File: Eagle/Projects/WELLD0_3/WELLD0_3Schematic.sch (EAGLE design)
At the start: 9 parts

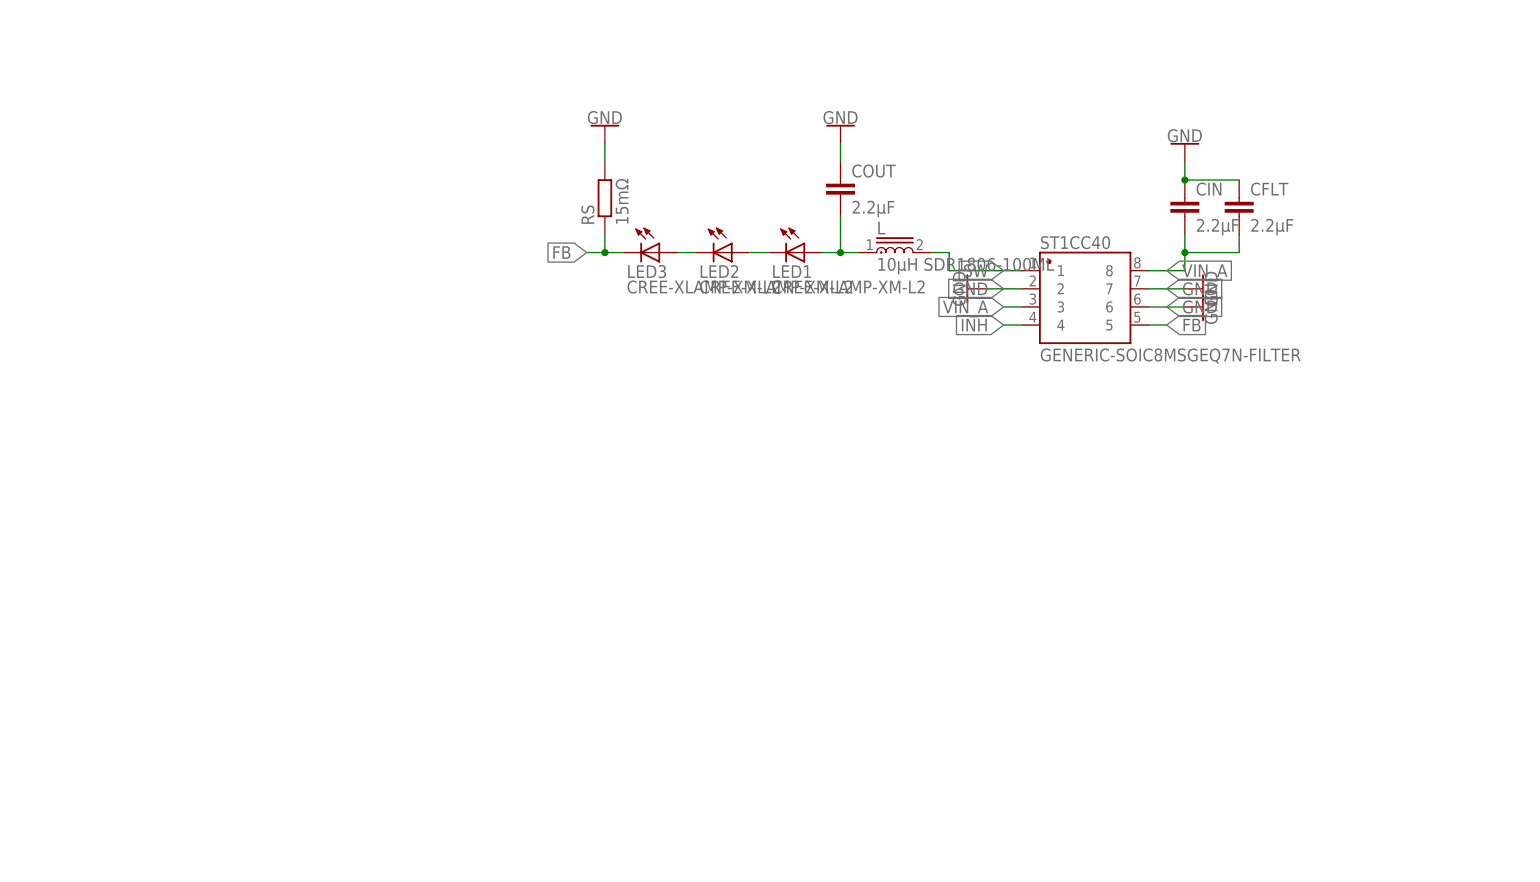
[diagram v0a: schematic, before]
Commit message: Work from 16/10-18
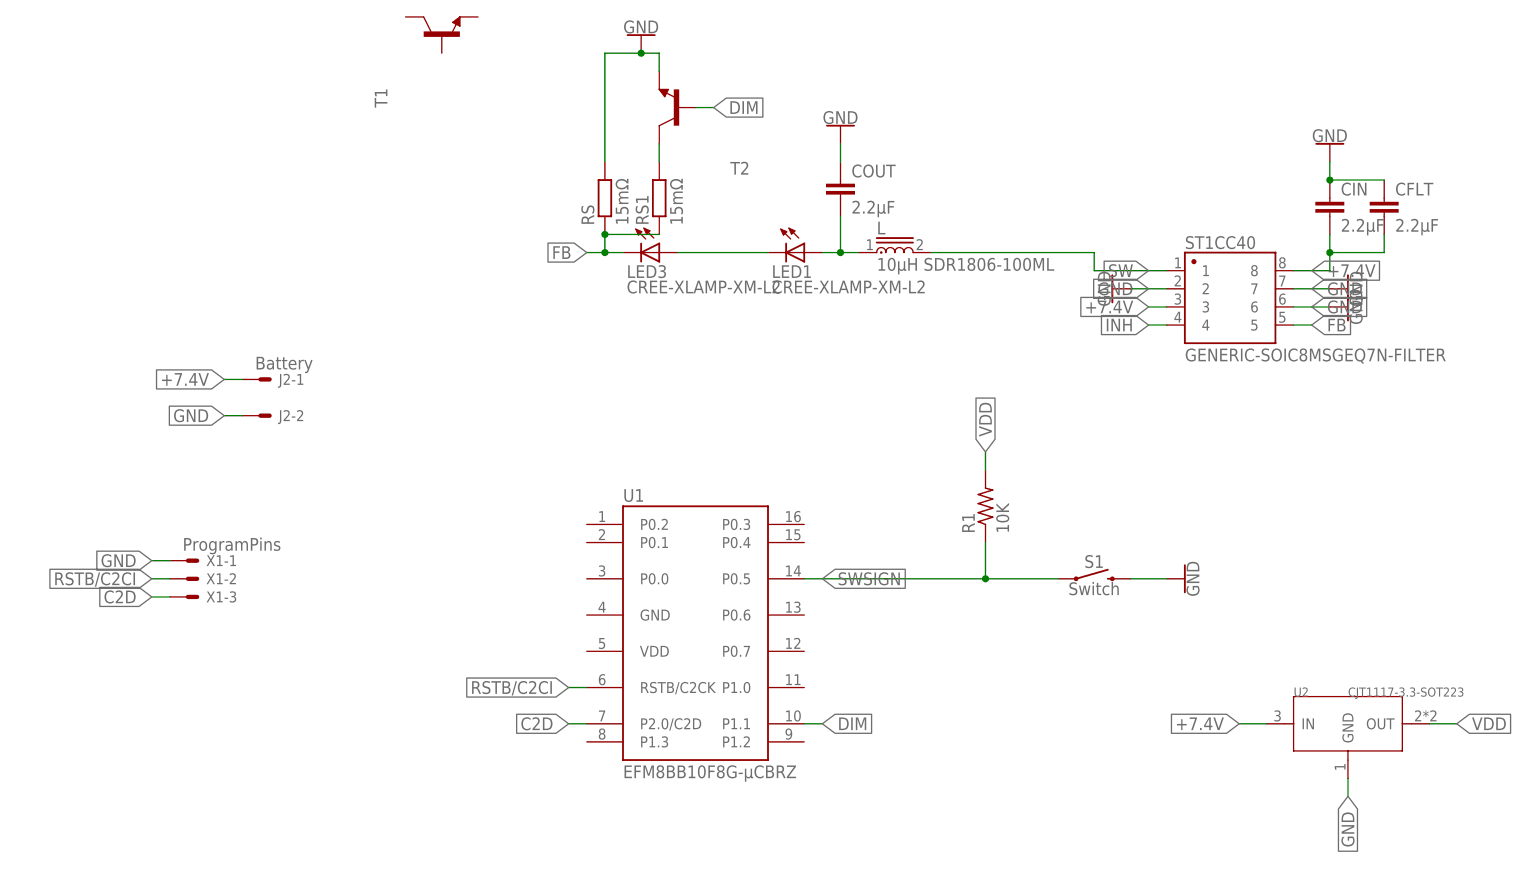
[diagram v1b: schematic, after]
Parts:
- removed LED2: CREE-XLAMP-XM-L2, led:CREE-XLAMP-XM-L
- added J2: Battery, con-molex:22-27-2021-02
- added R1: 10K, audio amplifier example:R-US_R0603
- added RS1: 15mΩ, rcl:R-EU_M1206
- added S1: Switch, SparkFun-Switches:MOMENTARY-SWITCH-SPST-SMD-6.2MM-TALL
- added T1, T2: (no value), DC_LOAD_AU:-NPN-SOT23-BEC
- added U1: EFM8BB10F8G-µCBRZ, adg451_adg452_adg453:EFM8BB10F8G-µCBRZ
- added U2: CJT1117-3.3-SOT223, Seeed-IC:PMIC-CJT1117-3.3(SOT223)
- added X1: ProgramPins, con-molex:C-GRID-03-70543
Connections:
- removed net VIN_A: CFLT.2, CIN.2, ST1CC40.3, ST1CC40.8
- new net +7.4V: CFLT.2, CIN.2, J2-1.S, ST1CC40.3, ST1CC40.8, U2.IN
- new net C2D: U1.P2.0/C2D, X1-3.S
- new net DIM: T2.B, U1.P1.1
- new net RSTB/C2CI: U1.RSTB/C2CK, X1-2.S
- new net SWSIGN: R1.1, S1.1, U1.P0.5
- new net VDD: R1.2, U2.OUT
- net FB: now also RS1.1
- net GND: now also J2-2.S, S1.2, T2.E, U2.GND, X1-1.S
- net N$2: now also LED3.A; no longer LED2.A
- net N$3: now also RS1.2, T2.C; no longer LED2.C, LED3.A
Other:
- moved on the sheet: CFLT, CIN, ST1CC40
